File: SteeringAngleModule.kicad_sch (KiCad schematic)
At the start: 18 parts, among them J1 Conn_01x03_Socket, J2 Conn_01x03_Socket, J3 Conn_01x04_Socket, U1 MCP3423

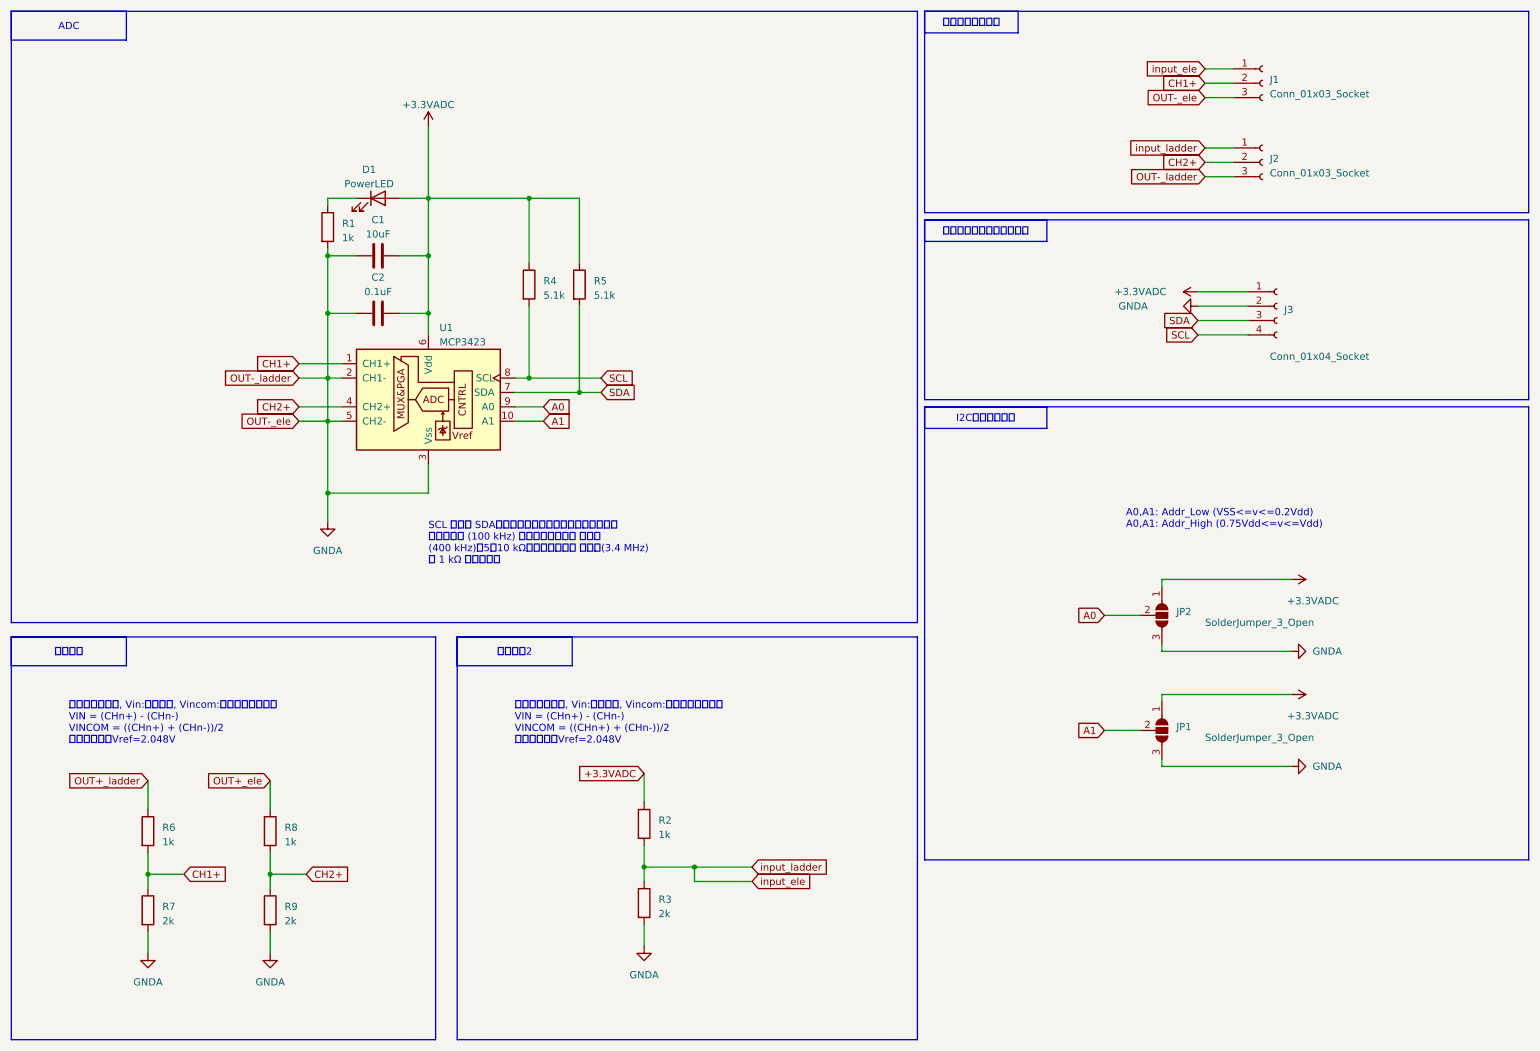
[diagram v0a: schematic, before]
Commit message: update
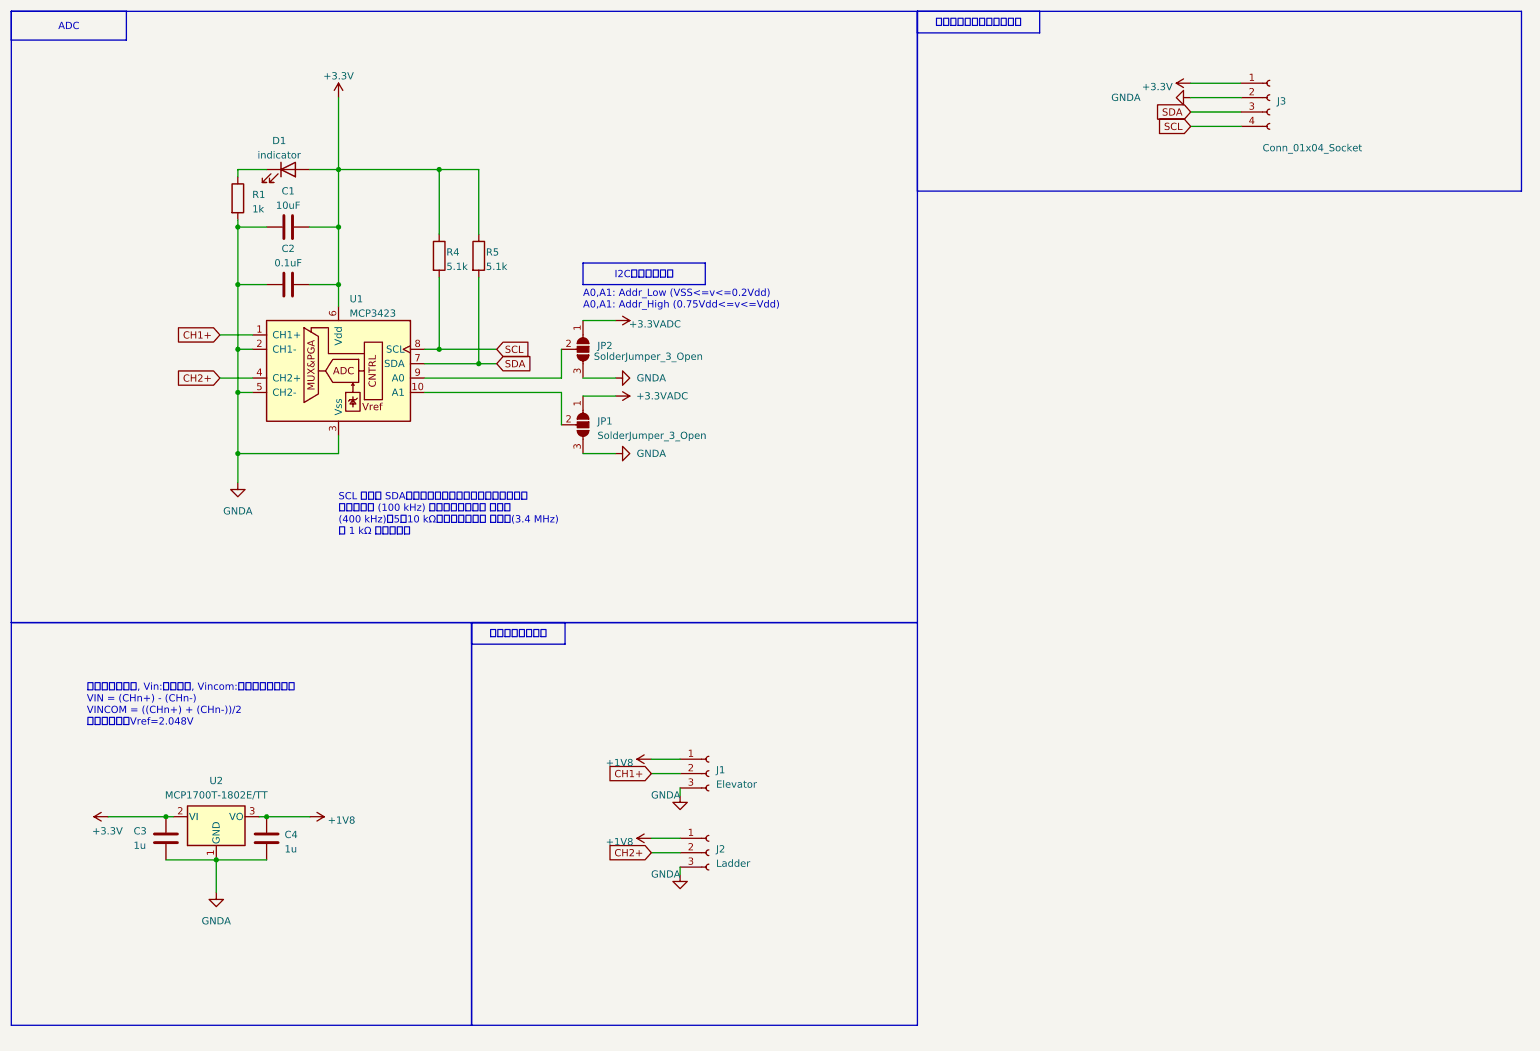
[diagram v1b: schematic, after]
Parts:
- removed R2, R6, R8: 1k, Resistor_SMD:R_0603_1608Metric, symbol Device:R
- removed R3, R7: 2k, Resistor_SMD:R_0603_1608Metric, symbol Device:R
- removed R9: 2k, symbol Device:R
- added C3, C4: 1u, symbol Device:C
- added U2: MCP1700T-1802E/TT, Package_TO_SOT_SMD:SOT-89-3, symbol Regulator_Linear:MCP1700x-180xxMB
- D1: value PowerLED -> indicator
- J1: value Conn_01x03_Socket -> Elevator
- J2: value Conn_01x03_Socket -> Ladder
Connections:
- net +3.3VADC: no longer C1.1, C2.1, D1.2 (A), J3.1 (Pin_1), R4.1, R5.1, U1.6 (Vdd)
- net GNDA: now also C3.2, C4.2, U2.1 (GND)
- net A0: no longer names the net of JP2.2 (C), U1.9 (A0)
- net A1: no longer names the net of JP1.2 (C), U1.10 (A1)
- net input_ele renamed +1V8
- net +1V8: now also C4.1, U2.3 (VO)
- new net +3.3V: C1.1, C2.1, C3.1, D1.2 (A), J3.1 (Pin_1), R4.1, R5.1, U1.6 (Vdd), U2.2 (VI)
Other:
- moved on the sheet: C1, C2, D1, J1, J2, J3, JP2, R1, R4, R5, U1
